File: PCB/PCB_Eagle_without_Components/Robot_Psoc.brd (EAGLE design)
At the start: 233.5 x 55.9 mm, 205 parts, among them U1 CY8C4247AZI-M485, U2 VCNL4010-GS08, U3 VCNL4010-GS08, U4 VCNL4010-GS08, U5 VCNL4010-GS08

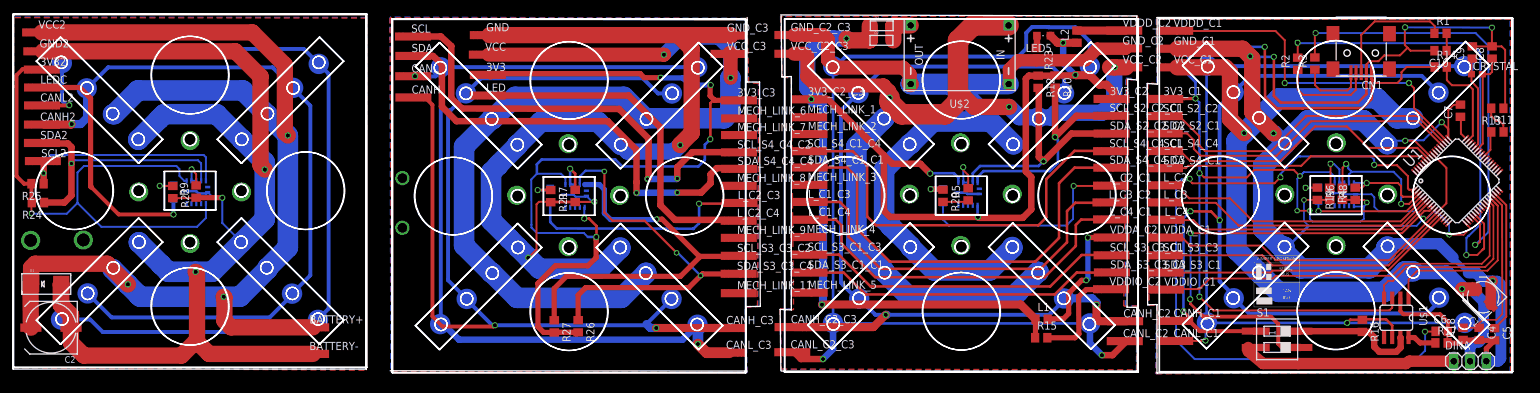
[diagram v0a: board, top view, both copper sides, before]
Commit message: 02/May/2017
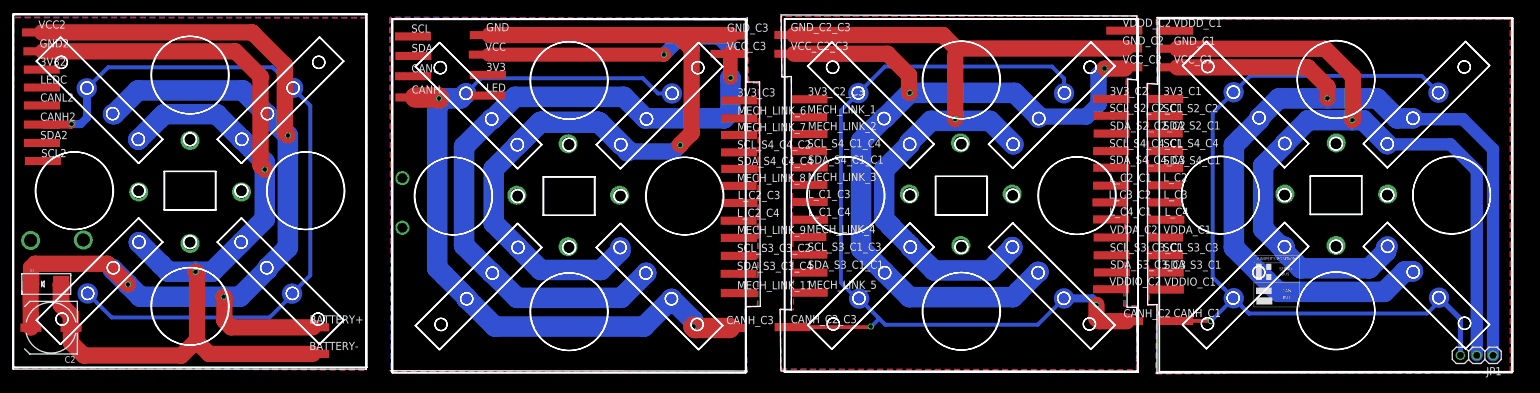
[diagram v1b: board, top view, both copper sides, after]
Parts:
- removed C1: (no value), rcl:UD-5X5,8_NICHICON
- removed C10: 0.1u, rcl:C0805
- removed C4: 2200pF, rcl:C0805
- removed C5: 10nF, rcl:C0805
- removed C6, C7: 1u, rcl:C0805
- removed C8: 36pF, rcl:C0805
- removed C9: 18pF, rcl:C0805
- removed CANL_1_C1, CANL_1_C2, CANL_1_C3, CANL_1_C4, CANL_2_C1, CANL_2_C2, CANL_2_C3, CANL_2_C4, CANL_3_C1, CANL_3_C2, CANL_3_C3, CANL_3_C4, CANL_4_C1, CANL_4_C2, CANL_4_C3, CANL_4_C4: TPB2,54, testpad:B2,54
- removed CANL_C1, CANL_C2, CANL_C2_C3, CANL_C3: PTR1TP11R, testpad:TP11R
- removed CN1: (no value), adafruit:USB-MINIB
- removed CRYSTAL: 32.768kHz, rcl:C0603
- removed D2, D3: (no value), adafruit:SOD-123
- removed DINA: (no value), pinhead:1X03
- removed L1, L2: 330-600Ohm@1Mhz, rcl:R0805
- removed LED1, LED2, LED3, LED4, LED5: (no value), adafruit:CHIPLED_0805
- removed R1, R11, R13, R15, R18, R2, R3: 0, rcl:R0805
- removed R10, R12, R14, R24, R25, R26, R27, R6, R8: 4.7k, rcl:R0805
- removed R16: 120, rcl:R0805
- removed R17: 10k, rcl:R0805
- removed R19, R20, R21, R22, R23, R4, R5, R7, R9: 220, rcl:R0805
- removed S1: SWS002, smd-special:SMS-002
- removed U$1: SN65HVD230/1, texas_instruments:SO8
- removed U$2: DC-DC-STEP-DOWN-MP2307, diy-modules:DC-DC-STEP-DOWN-MP2307
- removed U1: CY8C4247AZI-M485, CypressPSoC:TQFP64-10X10
- removed U2, U3, U4, U5: VCNL4010-GS08, VCNL4010-GS08:XDCR_VCNL4010-GS08
- added JP1: (no value), adafruit:1X03
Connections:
- removed net 3V3_C1: 3V3_C1.TP, CN1.VBUS, R14.1, R6.1, R8.1, U$1.3, U2.1, U2.7
- removed net 3V3_C2: 3V3_C2.TP, 3V3_C2_C3.TP, D2.C, D3.C, L1.1, L2.1, LED5.A, R10.1, R12.1, R15.1, U3.1, U3.7
- removed net 3V3_C3: 3V3.TP, 3V3_C3.TP, R26.2, R27.2, U4.1, U4.7
- removed net 3V3_C4: 3V32.TP, R24.2, R25.2, U5.1, U5.7
- removed net CANL: CANL_1_C1.TP, CANL_2_C1.TP, CANL_3_C1.TP, CANL_4_C1.TP, CANL_C1.TP, R16.1, U$1.6
- removed net CANL_C3: CANL.TP, CANL_1_C3.TP, CANL_2_C3.TP, CANL_3_C3.TP, CANL_4_C3.TP, CANL_C3.TP
- removed net CANL_C4: CANL2.TP, CANL_1_C4.TP, CANL_2_C4.TP, CANL_3_C4.TP, CANL_4_C4.TP
- removed net CAN_RX: U$1.4, U1.27
- removed net CAN_TX: U$1.1, U1.28
- removed net CMOD: C4.1, R18.2, U1.29
- removed net CTANK: C5.1, U1.30
- removed net DN_1: DINA.1, S1.2
- removed net LED_S1: LED1.A, U1.4
- removed net LED_S2: L_C2.TP, U1.5
- removed net LED_S2_C2: LED2.A, L_C2_C1.TP
- removed net LED_S3: L_C3.TP, U1.6
- removed net LED_S3_C3: LED3.A, L_C2_C3.TP
- removed net LED_S4: L_C4.TP, U1.7
- removed net LED_S4_C4: LED4.A, LEDC.TP
- removed net LED_T_S4: LED.TP, L_C2_C4.TP
- removed net MOTOR: S1.3, U1.8, U1.9
- removed net N$1: CN1.D+, R1.1
- removed net N$10: SDA_S3_C1_C1.TP, SDA_S3_C3_C3.TP
- removed net N$14: LED1.C, R19.1
- removed net N$15: LED2.C, R20.1
- removed net N$16: LED3.C, R21.1
- removed net N$17: LED4.C, R22.1
- removed net N$18: LED5.C, R23.1
- removed net N$2: CN1.ID, R2.1
- removed net N$20: L_C1_C4.TP, L_C4_C1.TP
- removed net N$21: R4.1, U2.2, U2.3
- removed net N$22: L_C1_C3.TP, L_C3_C2.TP
- removed net N$24: D2.A, D3.A, U$2.OUT+
- removed net N$26: SCL_S3_C1_C3.TP, SCL_S3_C3_C1.TP
- removed net N$27: SCL_S4_C1_C4.TP, SCL_S4_C4_C1.TP
- removed net N$3: CN1.GND, R3.1
- removed net N$32: CANL_1_C2.TP, CANL_2_C2.TP, CANL_3_C2.TP, CANL_4_C2.TP, CANL_C2.TP, CANL_C2_C3.TP
- removed net N$4: R11.2, R13.2
- removed net N$43: R5.2, U3.2, U3.3
- removed net N$44: SDA_S4_C1_C1.TP, SDA_S4_C4_C3.TP
- removed net N$46: R9.2, U5.2, U5.3
- removed net N$5: R16.2, S1.4, U$1.7
- removed net N$8: R7.2, U4.2, U4.3
- removed net N$9: R17.1, U$1.8
- removed net P0_1: R11.1, U1.40
- removed net P0_4: C8.1, CRYSTAL.2, U1.43
- removed net P0_5: C9.1, CRYSTAL.1, U1.44
- removed net SAR_BY: C6.1, U1.1
- removed net SCL_S1: R8.2, U1.2, U2.5
- removed net SCL_S2: SCL_S2_C2.TP, U1.51
- removed net SCL_S2_U: R10.2, SCL_S2_C2_C1.TP, U3.5
- removed net SCL_S3: SCL_S3_C3.TP, U1.12
- removed net SCL_S3_U: R27.1, SCL_S3_C3_C2.TP, U4.5
- removed net SCL_S4: SCL_S4_C4.TP, U1.58
- removed net SCL_S4_U: SCL.TP, SCL_S4_C4_C2.TP
- removed net SCL_S4_U_1: R25.1, SCL2.TP, U5.5
- removed net SDA_S1: R6.2, U1.3, U2.4
- removed net SDA_S2: SDA_S2_C1.TP, U1.52
- removed net SDA_S2_U: R12.2, SDA_S2_C2_C2.TP, U3.4
- removed net SDA_S3: SDA_S3_C1.TP, U1.13
- removed net SDA_S3_U: R26.1, SDA_S3_C3_C4.TP, U4.4
- removed net SDA_S4: SDA_S4_C1.TP, U1.59
- removed net SDA_S4_U: SDA.TP, SDA_S4_C4_C4.TP
- removed net SDA_S4_U_1: R24.1, SDA2.TP, U5.4
- removed net SWDCLK: R2.2, U1.21
- removed net SWDIO: R3.2, U1.20
- removed net UART_RX: U1.37
- removed net UART_TX: U1.38
- removed net VCCD: C7.1, U1.48
- removed net VDDA: U1.11, U1.56, VDDA_C1.TP
- removed net VDDA2: L1.2, VDDA_C2.TP
- removed net VDDD: U1.50, VDDD_C1.TP
- removed net VDDD2: L2.2, VDDD_C2.TP
- removed net VDDIO: U1.26, VDDIO_C1.TP
- removed net VDDIO2: R15.2, VDDIO_C2.TP
- removed net XRES: C10.1, R1.2, R14.2, U1.47
- net CANH: now also JP1.3; no longer S1.1
- net GND3: no longer R21.2, R7.1, U4.12, U4.13
- net GND4: no longer R22.2, R9.1, U5.12, U5.13
- net GND_C1: now also JP1.2; no longer C1.-, C10.2, C4.2, C5.2, C6.2, C7.2, C8.2, C9.2, CN1.D-, DINA.3, R13.1, R17.2, R18.1, R19.2, R4.2, U$1.2, U1.10, U1.17, U1.49, U1.57, U2.12, U2.13
- net GND_C2: no longer R20.2, R23.2, R5.1, U$2.IN-, U$2.OUT-, U3.12, U3.13
- net VCCC: now also JP1.1; no longer C1.+, DINA.2
- net VCC_C2: no longer U$2.IN+
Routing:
- net 3V3_C2: track 202.6 -> 0.00 mm, vias 7 -> 0
- net 3V3_C1: track 182.2 -> 0.00 mm, vias 8 -> 0
- net GND_C1: track 314.3 -> 138.1 mm, vias 11 -> 1
- net N$32: track 150.4 -> 0.00 mm, vias 2 -> 0
- net 3V3_C3: track 143.4 -> 0.00 mm, vias 5 -> 0
- net CANL_C3: track 138.5 -> 0.00 mm, vias 2 -> 0
- net CANL: track 138.2 -> 0.00 mm, vias 2 -> 0
- net CANL_C4: track 136.1 -> 0.00 mm, vias 1 -> 0
- net SAR_BY: track 113.3 -> 0.00 mm, vias 4 -> 0
- net 3V3_C4: track 83.8 -> 0.00 mm, vias 1 -> 0
- net MOTOR: track 73.8 -> 0.00 mm, vias 2 -> 0
- net SWDCLK: track 73.3 -> 0.00 mm, vias 2 -> 0
- net SCL_S4_U: track 71.3 -> 0.00 mm, vias 2 -> 0
- net SDA_S4_U: track 70.8 -> 0.00 mm, vias 2 -> 0
- net N$44: track 68.8 -> 0.00 mm
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
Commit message: 05/May
PCB
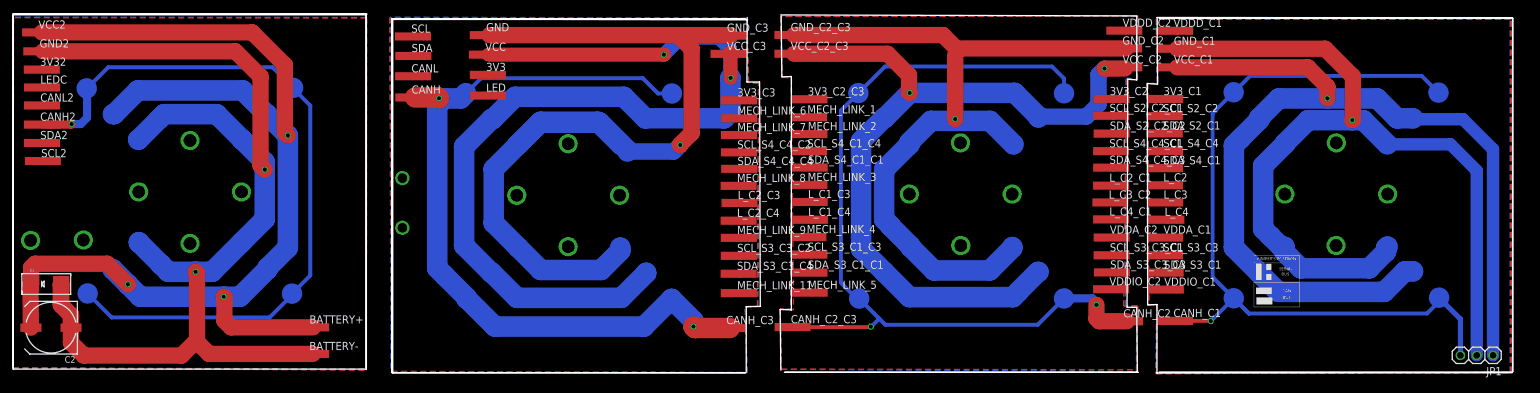
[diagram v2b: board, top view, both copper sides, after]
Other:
- outline, holes or cut-outs redrawn
